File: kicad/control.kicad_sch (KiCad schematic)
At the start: 14 parts, among them U10 74LS08, U11 74LS138, U2 74LS112, U8 74LS00, U9 74LS00

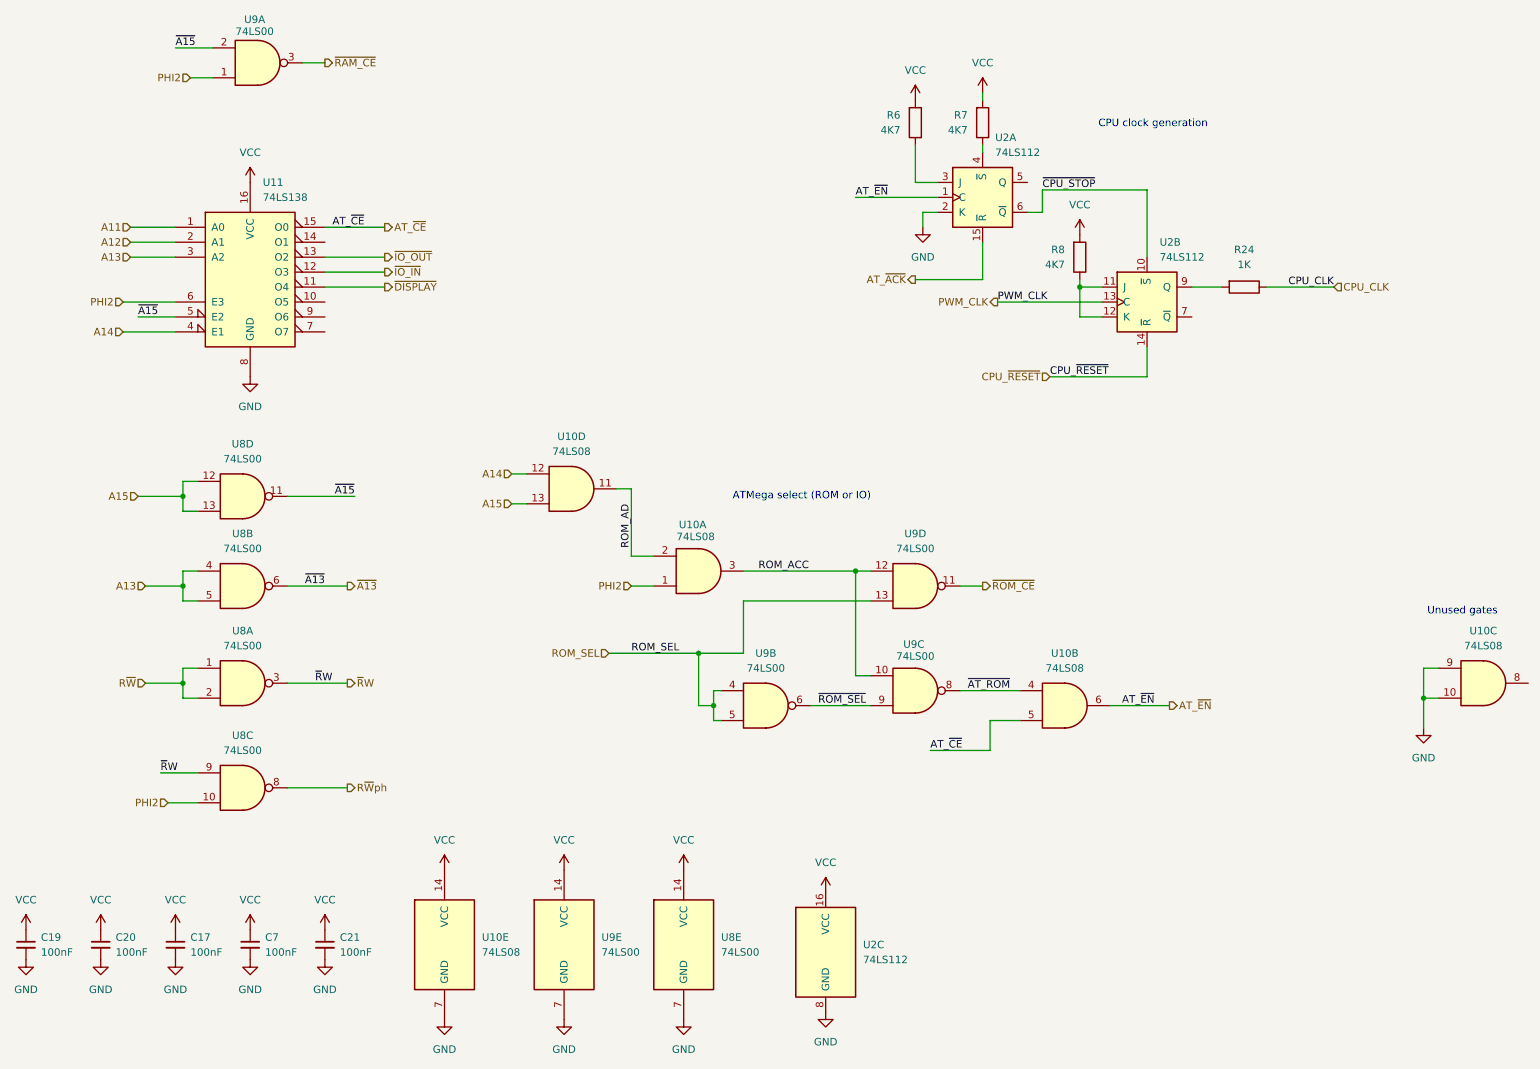
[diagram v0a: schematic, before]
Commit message: more updates for v1 rev2
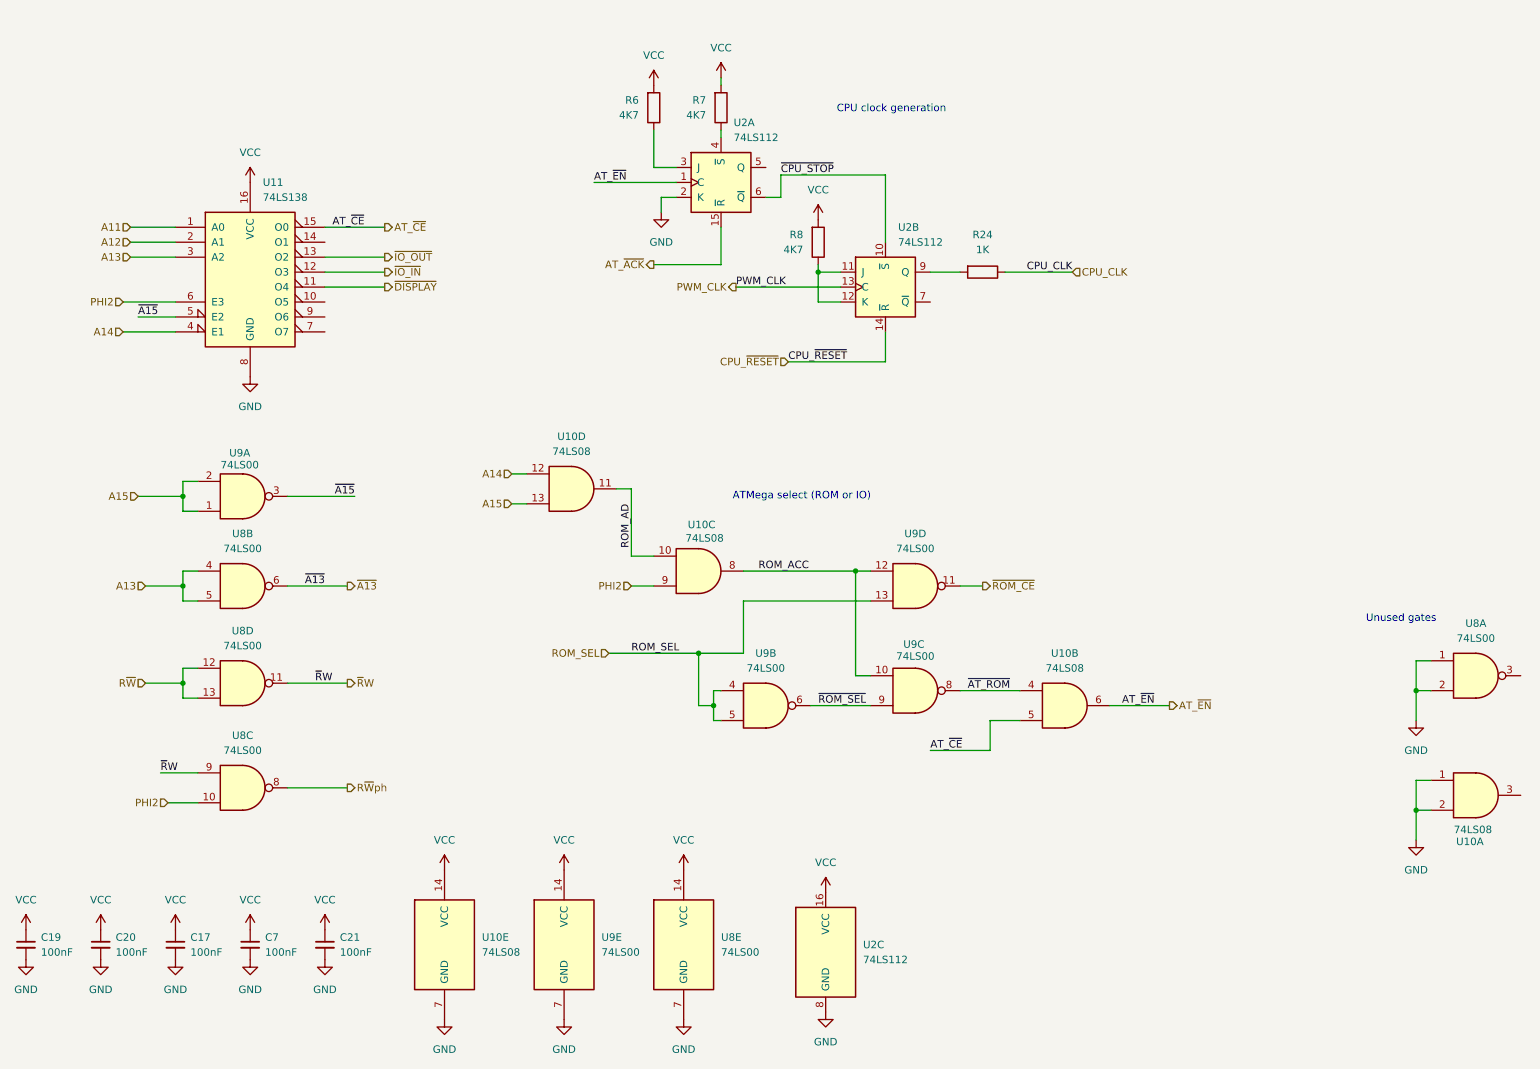
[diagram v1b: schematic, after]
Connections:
- net ~{RAM_CE} is gone; now on net ~{A15}: U9.3
- net A15: now also U9.1, U9.2; no longer U8.12, U8.13
- net GND: now also U10.1, U10.2, U8.1, U8.2; no longer U10.10, U10.9
- net PHI2: now also U10.9; no longer U10.1, U9.1
- net ROM_ACC: now also U10.8; no longer U10.3
- net ROM_AD: now also U10.10; no longer U10.2
- net R~{W}: now also U8.12, U8.13; no longer U8.1, U8.2
- net ~{A15}: no longer U8.11, U9.2
- net ~{R}W: now also U8.11; no longer U8.3
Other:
- moved on the sheet: R24, R6, R7, R8, U10A, U10C, U2A, U2B, U8A, U8D, U9A
